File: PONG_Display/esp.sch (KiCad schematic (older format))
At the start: 2 parts

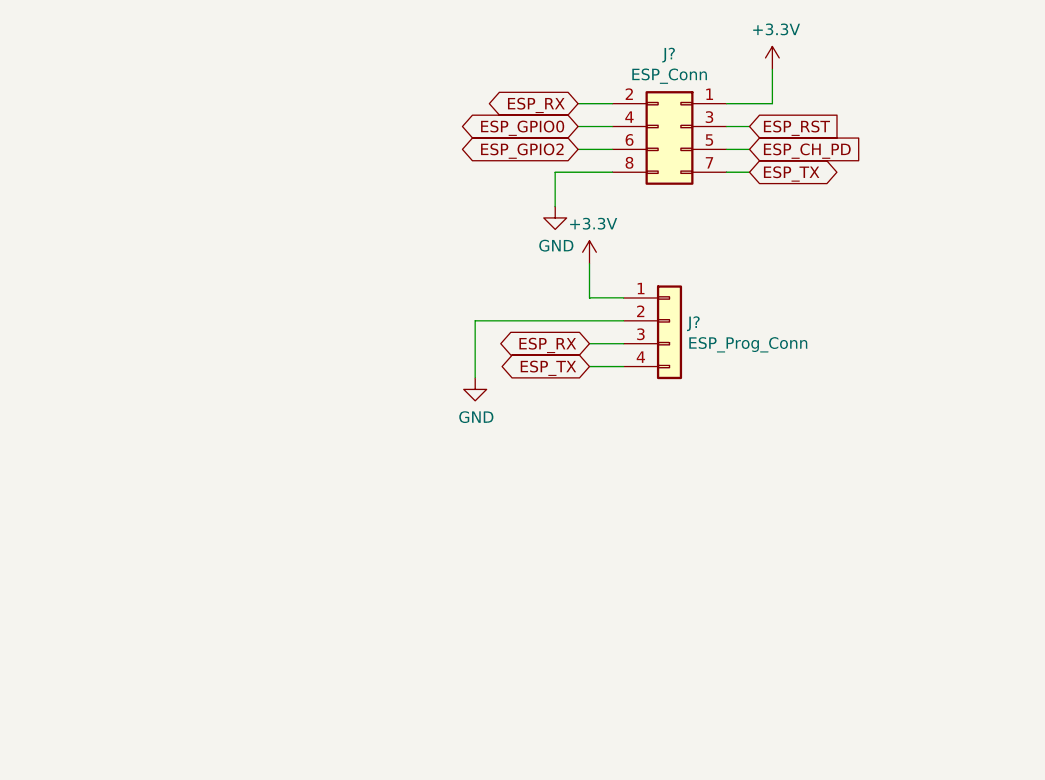
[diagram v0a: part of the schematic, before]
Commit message: V3
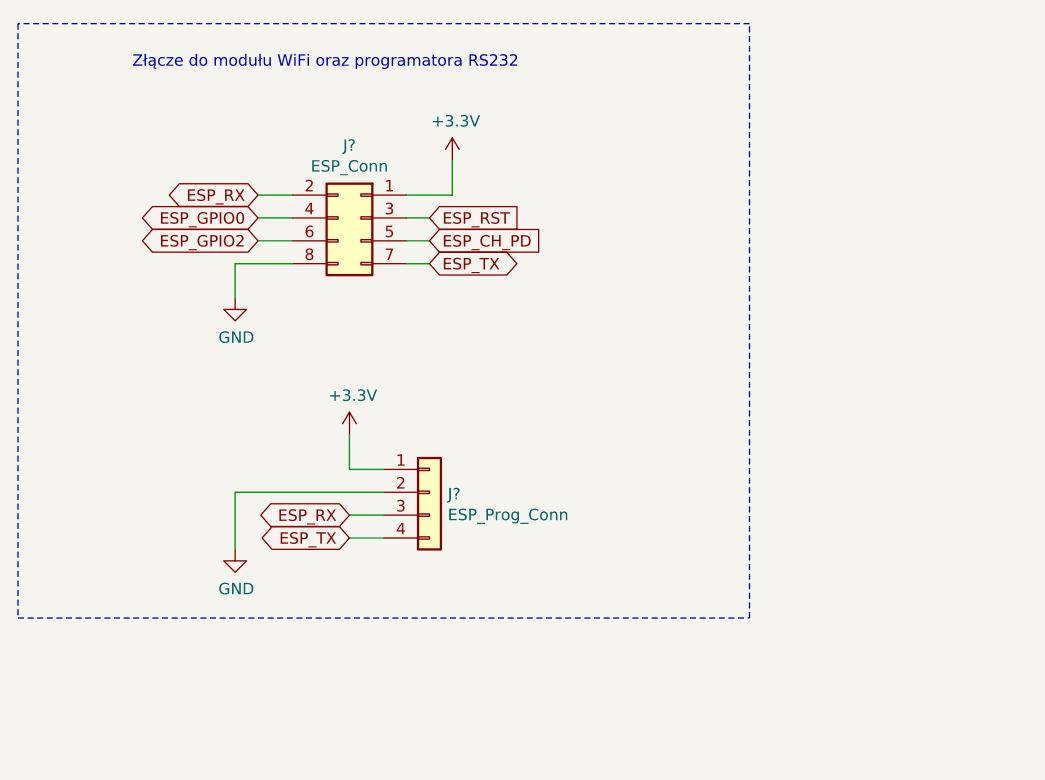
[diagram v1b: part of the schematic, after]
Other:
- note added: "Złącze do modułu WiFi oraz programatora RS232"
- moved on the sheet: J?
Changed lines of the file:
@@
 Comment4 ""
 $EndDescr
-Text GLabel 6100 1750 2    50   Input ~ 0
+Text GLabel 4700 2150 2    50   Input ~ 0
 ESP_RST
-Text GLabel 6100 1850 2    50   Input ~ 0
+Text GLabel 4700 2250 2    50   Input ~ 0
 ESP_CH_PD
-Text GLabel 6100 1950 2    50   BiDi ~ 0
+Text GLabel 4700 2350 2    50   BiDi ~ 0
 ESP_TX
-Text GLabel 5350 1650 0    50   BiDi ~ 0
+Text GLabel 3950 2050 0    50   BiDi ~ 0
 ESP_RX
-Text GLabel 5350 1750 0    50   BiDi ~ 0
+Text GLabel 3950 2150 0    50   BiDi ~ 0
 ESP_GPIO0
-Text GLabel 5350 1850 0    50   BiDi ~ 0
+Text GLabel 3950 2250 0    50   BiDi ~ 0
 ESP_GPIO2
 $Comp
 L Connector_Generic:Conn_02x04_Odd_Even J?
 U 1 1 5E838274
-P 5800 1750
+P 4400 2150
 AR Path="/5E80CCDD/5E838274" Ref="J?"  Part="1"
 AR Path="/5E80B1F8/5E838274" Ref="J?"  Part="1"
-F 0 "J?" H 5850 2067 50  0000 C CNN
-F 1 "ESP_Conn" H 5850 1976 50  0000 C CNN
-F 2 "" H 5800 1750 50  0001 C CNN
-F 3 "~" H 5800 1750 50  0001 C CNN
-	1    5800 1750
+F 0 "J?" H 4450 2467 50  0000 C CNN
+F 1 "ESP_Conn" H 4450 2376 50  0000 C CNN
+F 2 "" H 4400 2150 50  0001 C CNN
+F 3 "~" H 4400 2150 50  0001 C CNN
+	1    4400 2150
 	-1   0    0    -1
 $EndComp
 Wire Wire Line
-	6000 1750 6100 1750
+	4600 2150 4700 2150
 Wire Wire Line
-	6000 1850 6100 1850
+	4600 2250 4700 2250
 Wire Wire Line
-	6000 1950 6100 1950
+	4600 2350 4700 2350
 Wire Wire Line
-	5350 1650 5500 1650
+	3950 2050 4100 2050
 Wire Wire Line
-	5350 1750 5500 1750
+	3950 2150 4100 2150
 Wire Wire Line
-	5500 1850 5350 1850
+	4100 2250 3950 2250
 $Comp
 L Connector_Generic:Conn_01x04 J?
 U 1 1 5E838282
-P 5750 2600
+P 4700 3350
 AR Path="/5E80CCDD/5E838282" Ref="J?"  Part="1"
 AR Path="/5E80B1F8/5E838282" Ref="J?"  Part="1"
-F 0 "J?" H 5830 2592 50  0000 L CNN
-F 1 "ESP_Prog_Conn" H 5830 2501 50  0000 L CNN
-F 2 "" H 5750 2600 50  0001 C CNN
-F 3 "~" H 5750 2600 50  0001 C CNN
-	1    5750 2600
+F 0 "J?" H 4780 3342 50  0000 L CNN
+F 1 "ESP_Prog_Conn" H 4780 3251 50  0000 L CNN
+F 2 "" H 4700 3350 50  0001 C CNN
+F 3 "~" H 4700 3350 50  0001 C CNN
+	1    4700 3350
 	1    0    0    -1
 $EndComp
 Wire Wire Line
-	5400 2500 5550 2500
+	4350 3250 4500 3250
 Wire Wire Line
-	5400 2700 5550 2700
+	4350 3450 4500 3450
 Wire Wire Line
-	5400 2800 5550 2800
-Text GLabel 5400 2800 0    50   BiDi ~ 0
+	4350 3550 4500 3550
+Text GLabel 4350 3550 0    50   BiDi ~ 0
 ESP_TX
-Text GLabel 5400 2700 0    50   BiDi ~ 0
+Text GLabel 4350 3450 0    50   BiDi ~ 0
 ESP_RX
 Text Notes 7800 7500 0    50   ~ 0
 Schemat modułu WiFi
 $Comp
-L power:+3.3V #PWR?
+L power:+3.3V #PWR0173
 U 1 1 5E858E36
-P 6200 1500
-F 0 "#PWR?" H 6200 1350 50  0001 C CNN
-F 1 "+3.3V" H 6215 1673 50  0000 C CNN
-F 2 "" H 6200 1500 50  0001 C CNN
-F 3 "" H 6200 1500 50  0001 C CNN
-	1    6200 1500
+P 4800 1900
+F 0 "#PWR0173" H 4800 1750 50  0001 C CNN
+F 1 "+3.3V" H 4815 2073 50  0000 C CNN
+F 2 "" H 4800 1900 50  0001 C CNN
+F 3 "" H 4800 1900 50  0001 C CNN
+	1    4800 1900
 	1    0    0    -1
 $EndComp
 $Comp
-L power:GND #PWR?
+L power:GND #PWR0174
 U 1 1 5E85942E
-P 5250 2100
-F 0 "#PWR?" H 5250 1850 50  0001 C CNN
-F 1 "GND" H 5255 1927 50  0000 C CNN
-F 2 "" H 5250 2100 50  0001 C CNN
-F 3 "" H 5250 2100 50  0001 C CNN
-	1    5250 2100
+P 3850 2500
+F 0 "#PWR0174" H 3850 2250 50  0001 C CNN
+F 1 "GND" H 3855 2327 50  0000 C CNN
+F 2 "" H 3850 2500 50  0001 C CNN
+F 3 "" H 3850 2500 50  0001 C CNN
+	1    3850 2500
 	1    0    0    -1
 $EndComp
 Wire Wire Line
-	6200 1500 6200 1650
+	4800 1900 4800 2050
 Wire Wire Line
-	6000 1650 6200 1650
+	4600 2050 4800 2050
 Wire Wire Line
-	5250 1950 5250 2100
+	3850 2350 3850 2500
 Wire Wire Line
-	5250 1950 5500 1950
+	3850 2350 4100 2350
 $Comp
-L power:+3.3V #PWR?
+L power:+3.3V #PWR0175
 U 1 1 5E859CE6
-P 5400 2350
-F 0 "#PWR?" H 5400 2200 50  0001 C CNN
-F 1 "+3.3V" H 5415 2523 50  0000 C CNN
-F 2 "" H 5400 2350 50  0001 C CNN
-F 3 "" H 5400 2350 50  0001 C CNN
-	1    5400 2350
+P 4350 3100
+F 0 "#PWR0175" H 4350 2950 50  0001 C CNN
+F 1 "+3.3V" H 4365 3273 50  0000 C CNN
+F 2 "" H 4350 3100 50  0001 C CNN
+F 3 "" H 4350 3100 50  0001 C CNN
+	1    4350 3100
 	1    0    0    -1
 $EndComp
 $Comp
-L power:GND #PWR?
+L power:GND #PWR0176
 U 1 1 5E85A6F5
-P 4900 2850
-F 0 "#PWR?" H 4900 2600 50  0001 C CNN
-F 1 "GND" H 4905 2677 50  0000 C CNN
-F 2 "" H 4900 2850 50  0001 C CNN
-F 3 "" H 4900 2850 50  0001 C CNN
-	1    4900 2850
+P 3850 3600
+F 0 "#PWR0176" H 3850 3350 50  0001 C CNN
+F 1 "GND" H 3855 3427 50  0000 C CNN
+F 2 "" H 3850 3600 50  0001 C CNN
+F 3 "" H 3850 3600 50  0001 C CNN
+	1    3850 3600
 	1    0    0    -1
 $EndComp
 Wire Wire Line
-	5400 2350 5400 2500
+	4350 3100 4350 3250
 Wire Wire Line
-	4900 2600 4900 2850
+	3850 3350 3850 3600
 Wire Wire Line
-	4900 2600 5550 2600
+	3850 3350 4500 3350
+Wire Notes Line
+	2900 3900 6100 3900
+Wire Notes Line
+	6100 3900 6100 1300
+Wire Notes Line
+	6100 1300 2900 1300
+Wire Notes Line
+	2900 1300 2900 3900
+Text Notes 3400 1500 0    50   ~ 0
+Złącze do modułu WiFi oraz programatora RS232
 $EndSCHEMATC
